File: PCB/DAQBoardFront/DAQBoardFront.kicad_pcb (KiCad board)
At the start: 2 copper layers, 94 x 68 mm, 14 parts, among them J2 53375-0410

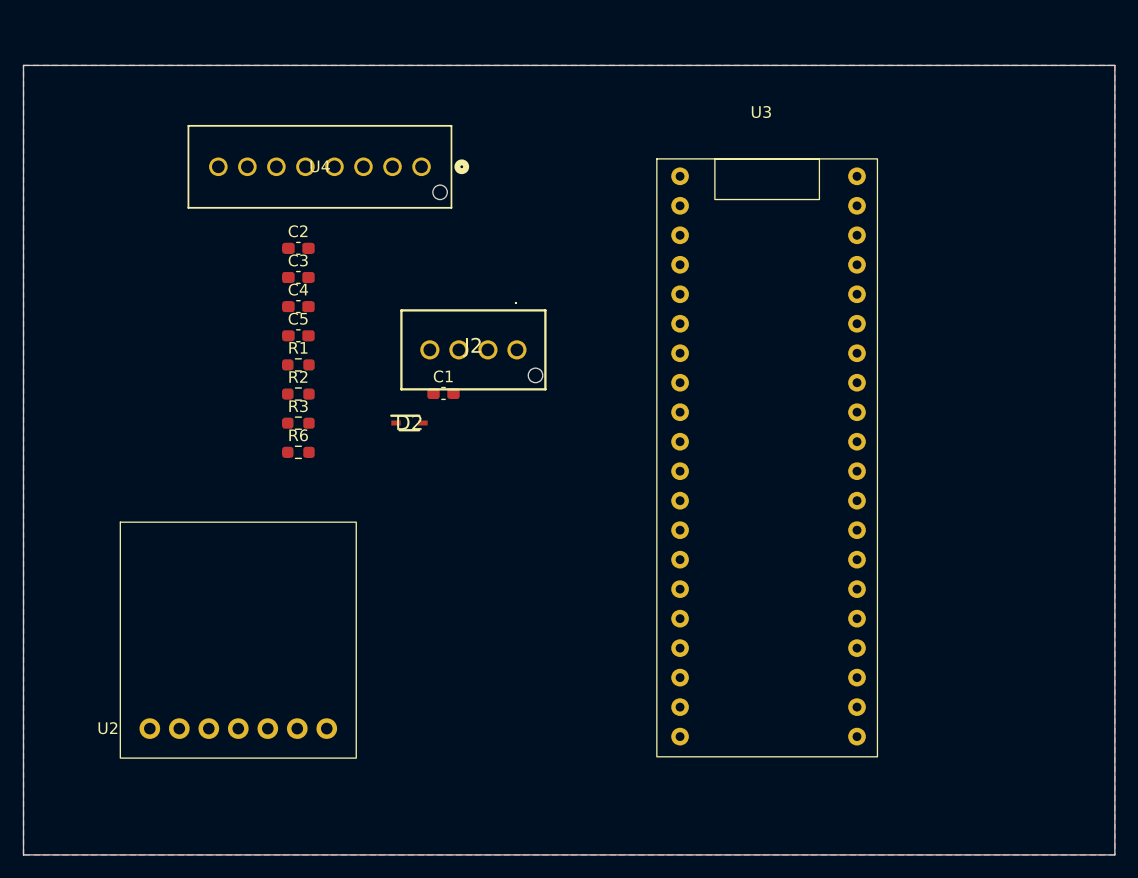
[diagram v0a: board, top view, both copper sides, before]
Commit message: Version 1.0 completed
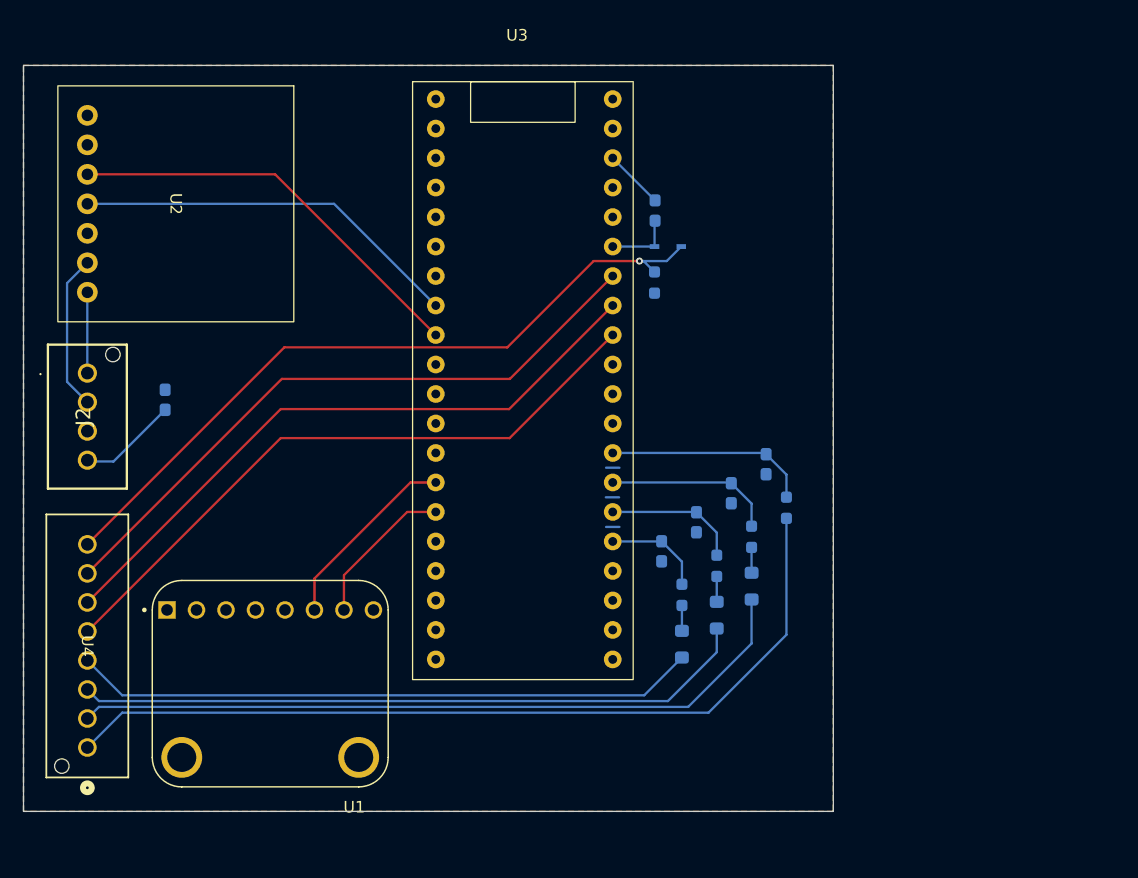
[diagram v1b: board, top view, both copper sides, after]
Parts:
- added L1: 10u, Inductor_SMD:L_0805_2012Metric_Pad1.05x1.20mm_HandSolder, B.Cu at (155.2, 113.3)
- added L2: 10u, Inductor_SMD:L_0805_2012Metric_Pad1.05x1.20mm_HandSolder, B.Cu at (158.2, 110.8)
- added L3: L, Inductor_SMD:L_0805_2012Metric_Pad1.05x1.20mm_HandSolder, B.Cu at (161.2, 108.3)
- added R4: 24k, LED_SMD:LED_0603_1608Metric_Pad1.05x0.95mm_HandSolder, B.Cu at (152.9, 76.0)
- added R5: 2k, Resistor_SMD:R_0603_1608Metric_Pad0.98x0.95mm_HandSolder, B.Cu at (152.8, 82.2)
- added U1: ~, CFR-Footprint-Library:MODULE_2019, F.Cu at (119.8, 116.8)
- C1, C2, C3, C4, C5, D2, R1, R2, R3, R6: moved to B.Cu
- moved U4 57.7 mm to (104.0, 122.2), turned to -90 degrees
- moved U2 53.1 mm to (104.0, 67.8), turned to -90 degrees
- moved R6 42.3 mm to (164.2, 101.6), turned to -90 degrees
- moved C5 41.8 mm to (162.5, 97.8), turned to -90 degrees
- moved C2 40.7 mm to (153.5, 105.3), turned to -90 degrees
- moved C4 40.6 mm to (159.5, 100.3), turned to -90 degrees
- moved C3 40.2 mm to (156.5, 102.8), turned to -90 degrees
- moved R3 40.2 mm to (161.2, 104.1), turned to -90 degrees
- moved R2 39.0 mm to (158.2, 106.6), turned to -90 degrees
- moved R1 38.5 mm to (155.2, 109.1), turned to -90 degrees
- moved J2 37.1 mm to (104.0, 90.0), turned to 90 degrees
- moved D2 27.0 mm to (154.0, 79.1), turned to 180 degrees
- moved C1 24.0 mm to (110.7, 92.3), turned to 90 degrees
- moved U3 22.1 mm to (134.0, 66.4)
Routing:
- net /ExtraAnalog: track 0.00 -> 74.3 mm
- net /SteeringAngle: track 0.00 -> 63.7 mm
- net /Brake P Input: track 0.00 -> 63.5 mm, vias 0 -> 1
- net /FLSus: track 0.00 -> 58.4 mm
- net /FLHallEffect: track 0.00 -> 55.9 mm
- net /FRHallEffect: track 0.00 -> 55.8 mm
- net /ExtraDigital: track 0.00 -> 55.8 mm
- net /FRSus: track 0.00 -> 53.8 mm
- net /CANTx: track 0.00 -> 35.7 mm
- net /CANRx: track 0.00 -> 33.6 mm
- net Net-(U3-A3): track 0.00 -> 17.7 mm
- net /Acc SCL: track 0.00 -> 16.6 mm
- net Net-(U3-A2): track 0.00 -> 14.7 mm
- net /+3.3V: track 0.00 -> 13.7 mm
- net /CAN Hi: track 0.00 -> 13.4 mm
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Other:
- board size 94 x 68 mm -> 69.8 x 64.2 mm
